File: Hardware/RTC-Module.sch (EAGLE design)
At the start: 18 parts, among them J4 455-1750-1-ND

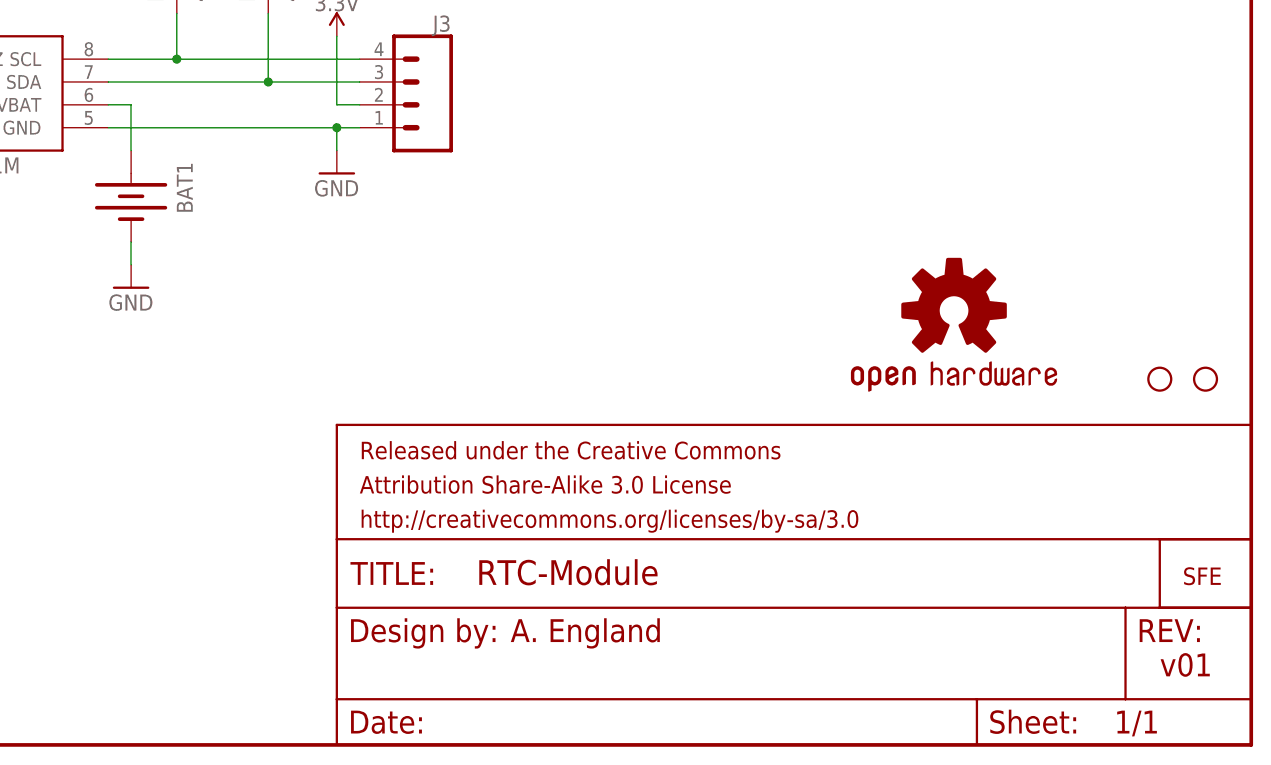
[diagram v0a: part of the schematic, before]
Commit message: Board ready for design review
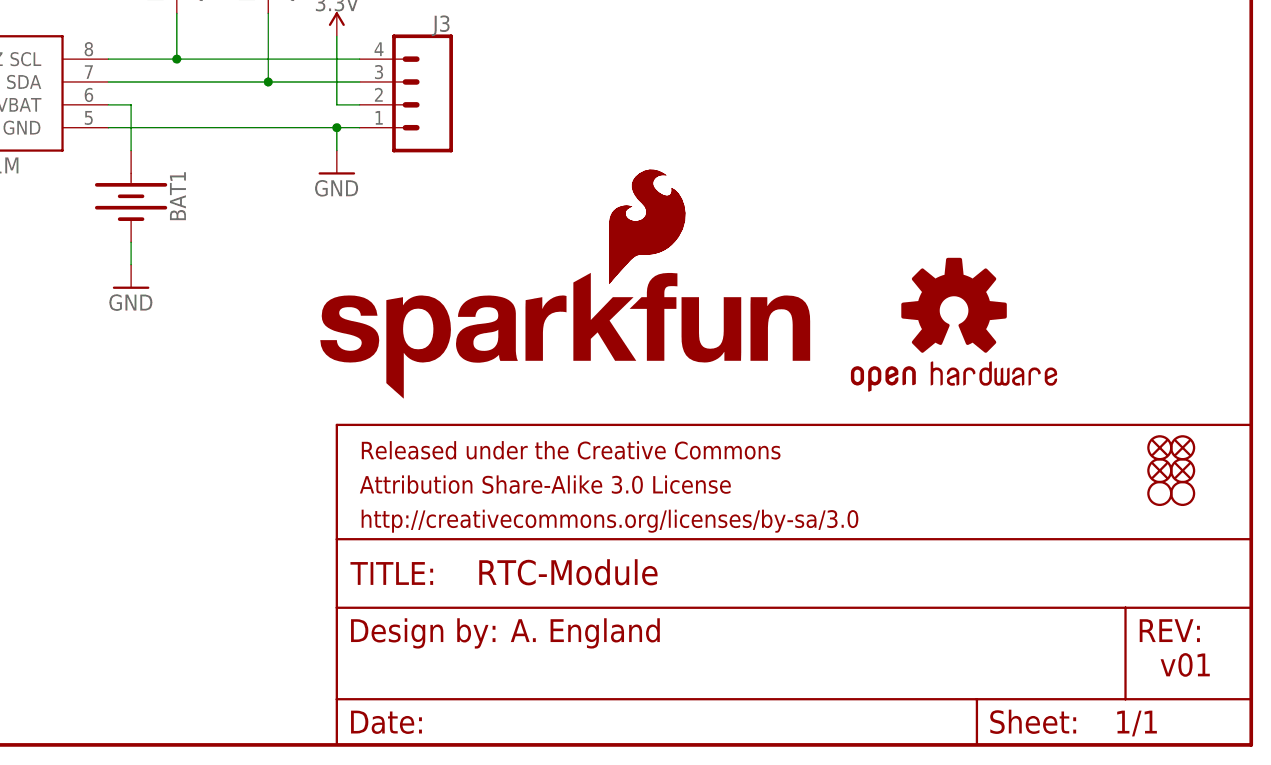
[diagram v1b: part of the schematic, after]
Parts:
- removed U$2: LOGO-SFESK, SparkFun:LOGO-SFESK
- added FD1, FD2, FD3, FD4: FIDUCIALUFIDUCIAL, SparkFun-Aesthetics:FIDUCIALUFIDUCIAL
- added LOGO2: SFE_LOGO_FLAME.1_INCH, SparkFun-Aesthetics:SFE_LOGO_FLAME.1_INCH
- added LOGO3: SFE_LOGO_NAME_FLAME.1_INCH, SparkFun-Aesthetics:SFE_LOGO_NAME_FLAME.1_INCH
- BAT1: device SparkFun-Electromechanical:BATTERY12PTH -> SparkFun-Batteries:BATTERY-12MM_PTH
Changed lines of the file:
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@@
 </classes>
 <parts>
-<part name="U$2" library="SparkFun" deviceset="LOGO-SFE" device="SK"/>
 <part name="U$6" library="SparkFun" deviceset="STAND-OFF" device=""/>
 <part name="U$7" library="SparkFun" deviceset="STAND-OFF" device=""/>
-<part name="BAT1" library="SparkFun-Electromechanical" deviceset="BATTERY" device="12PTH"/>
+<part name="BAT1" library="SparkFun-Batteries" deviceset="BATTERY" device="-12MM_PTH"/>
 <part name="C1" library="SparkFun-Capacitors" deviceset="0.1UF-25V(+80/-20%)(0603)" device="" value="0.1uF"/>
 <part name="GND2" library="SparkFun" deviceset="GND" device=""/>
@@
 <part name="SUPPLY5" library="SparkFun-PowerSymbols" deviceset="3.3V" device=""/>
 <part name="J4" library="SparkFun-Connectors" deviceset="CONN_03" device="" value="455-1750-1-ND"/>
+<part name="LOGO2" library="SparkFun-Aesthetics" deviceset="SFE_LOGO_FLAME" device=".1_INCH"/>
+<part name="LOGO3" library="SparkFun-Aesthetics" deviceset="SFE_LOGO_NAME_FLAME" device=".1_INCH"/>
+<part name="FD1" library="SparkFun-Aesthetics" deviceset="FIDUCIAL" device="UFIDUCIAL"/>
+<part name="FD2" library="SparkFun-Aesthetics" deviceset="FIDUCIAL" device="UFIDUCIAL"/>
+<part name="FD3" library="SparkFun-Aesthetics" deviceset="FIDUCIAL" device="UFIDUCIAL"/>
+<part name="FD4" library="SparkFun-Aesthetics" deviceset="FIDUCIAL" device="UFIDUCIAL"/>
 </parts>
 <sheets>
@@
 </plain>
 <instances>
-<instance part="U$2" gate="G$1" x="241.3" y="17.78"/>
-<instance part="U$6" gate="G$1" x="238.76" y="40.64"/>
-<instance part="U$7" gate="G$1" x="243.84" y="40.64"/>
+<instance part="U$6" gate="G$1" x="238.76" y="27.94"/>
+<instance part="U$7" gate="G$1" x="241.3" y="27.94"/>
 <instance part="BAT1" gate="G$1" x="124.46" y="60.96" rot="R270"/>
 <instance part="C1" gate="G$1" x="45.72" y="78.74"/>
@@
 <instance part="SUPPLY5" gate="G$1" x="81.28" y="101.6"/>
 <instance part="J4" gate="J$1" x="76.2" y="22.86"/>
+<instance part="LOGO2" gate="G$1" x="177.2158" y="50.6984"/>
+<instance part="LOGO3" gate="G$1" x="144.78" y="38.1"/>
+<instance part="FD1" gate="G$1" x="238.76" y="33.02"/>
+<instance part="FD2" gate="G$1" x="241.3" y="33.02"/>
+<instance part="FD3" gate="G$1" x="241.3" y="30.48"/>
+<instance part="FD4" gate="G$1" x="238.76" y="30.48"/>
 </instances>
 <busses>
